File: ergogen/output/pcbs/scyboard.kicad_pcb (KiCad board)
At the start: 2 copper layers, 148.5 x 100.9 mm, 76 parts

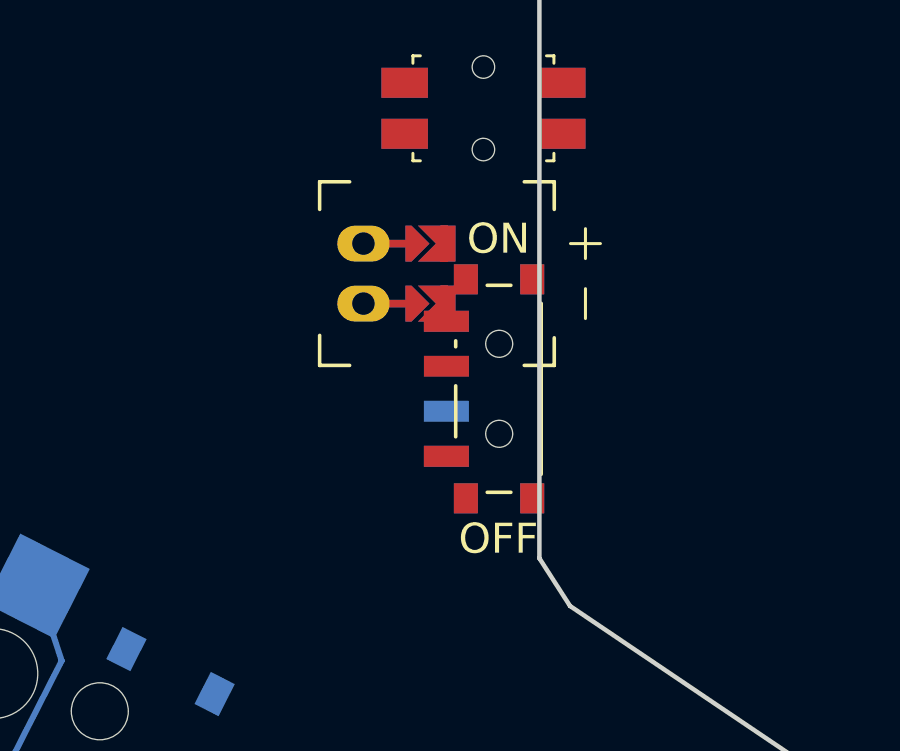
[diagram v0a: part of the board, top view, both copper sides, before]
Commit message: Compile
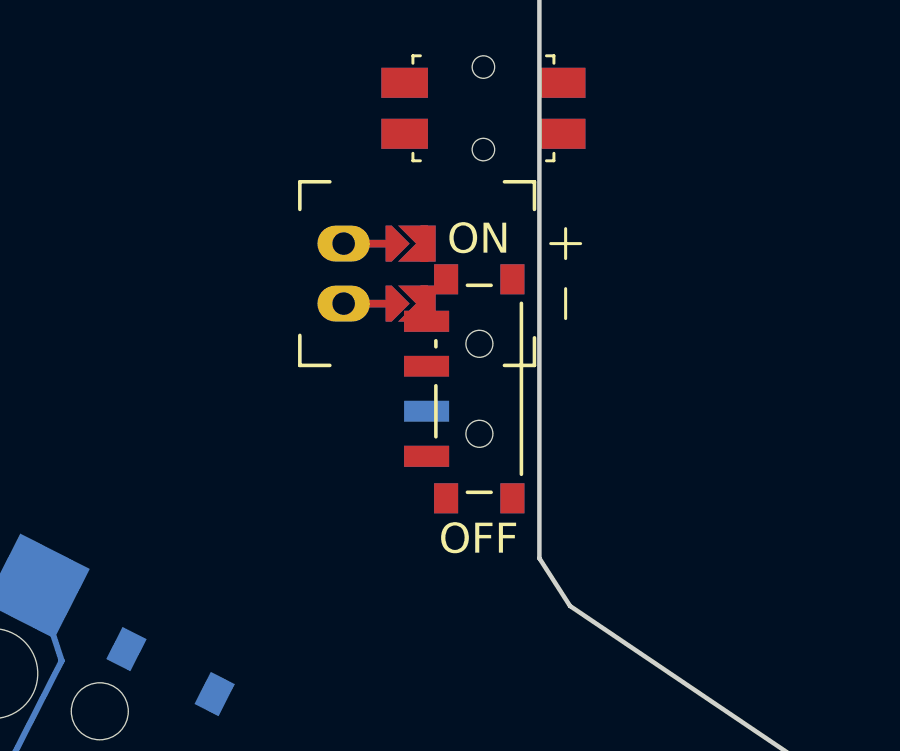
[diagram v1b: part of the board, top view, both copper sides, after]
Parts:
- moved JST1 0.66 mm to (163.2, 89.0)
- moved PWR1 0.66 mm to (167.7, 92.9)
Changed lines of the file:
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@@
   (footprint "ceoloide:power_switch_smd_side"
     (layer "F.Cu")
-    (at 168.385 92.87 0)
+    (at 167.725 92.87 0)
     (property "Reference" "PWR1"
       (at -3.6 0 -90)
@@
     (footprint "ceoloide:battery_connector_jst_ph_2"
         (layer "F.Cu")
-        (at 163.885 89.03 90)
+        (at 163.225 89.03 90)
         (property "Reference" "JST1"
             (at 0 4.8 90)
@@
         )
     )
-    (segment (start 165.685 90.03) (end 163.885 90.03) (width 0.25) (layer "F.Cu") (net 75))
-    (segment (start 165.685 90.03) (end 163.885 90.03) (width 0.25) (layer "B.Cu") (net 75))
-    (segment (start 165.685 88.03) (end 163.885 88.03) (width 0.25) (layer "F.Cu") (net 76))
-    (segment (start 165.685 88.03) (end 163.885 88.03) (width 0.25) (layer "B.Cu") (net 76))
+    (segment (start 165.025 90.03) (end 163.225 90.03) (width 0.25) (layer "F.Cu") (net 75))
+    (segment (start 165.025 90.03) (end 163.225 90.03) (width 0.25) (layer "B.Cu") (net 75))
+    (segment (start 165.025 88.03) (end 163.225 88.03) (width 0.25) (layer "F.Cu") (net 76))
+    (segment (start 165.025 88.03) (end 163.225 88.03) (width 0.25) (layer "B.Cu") (net 76))
   (footprint "ceoloide:mounting_hole_npth"
     (layer "F.Cu")
